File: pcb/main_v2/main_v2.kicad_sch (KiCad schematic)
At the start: 1 part, among them J102 Conn_02x06_Odd_Even

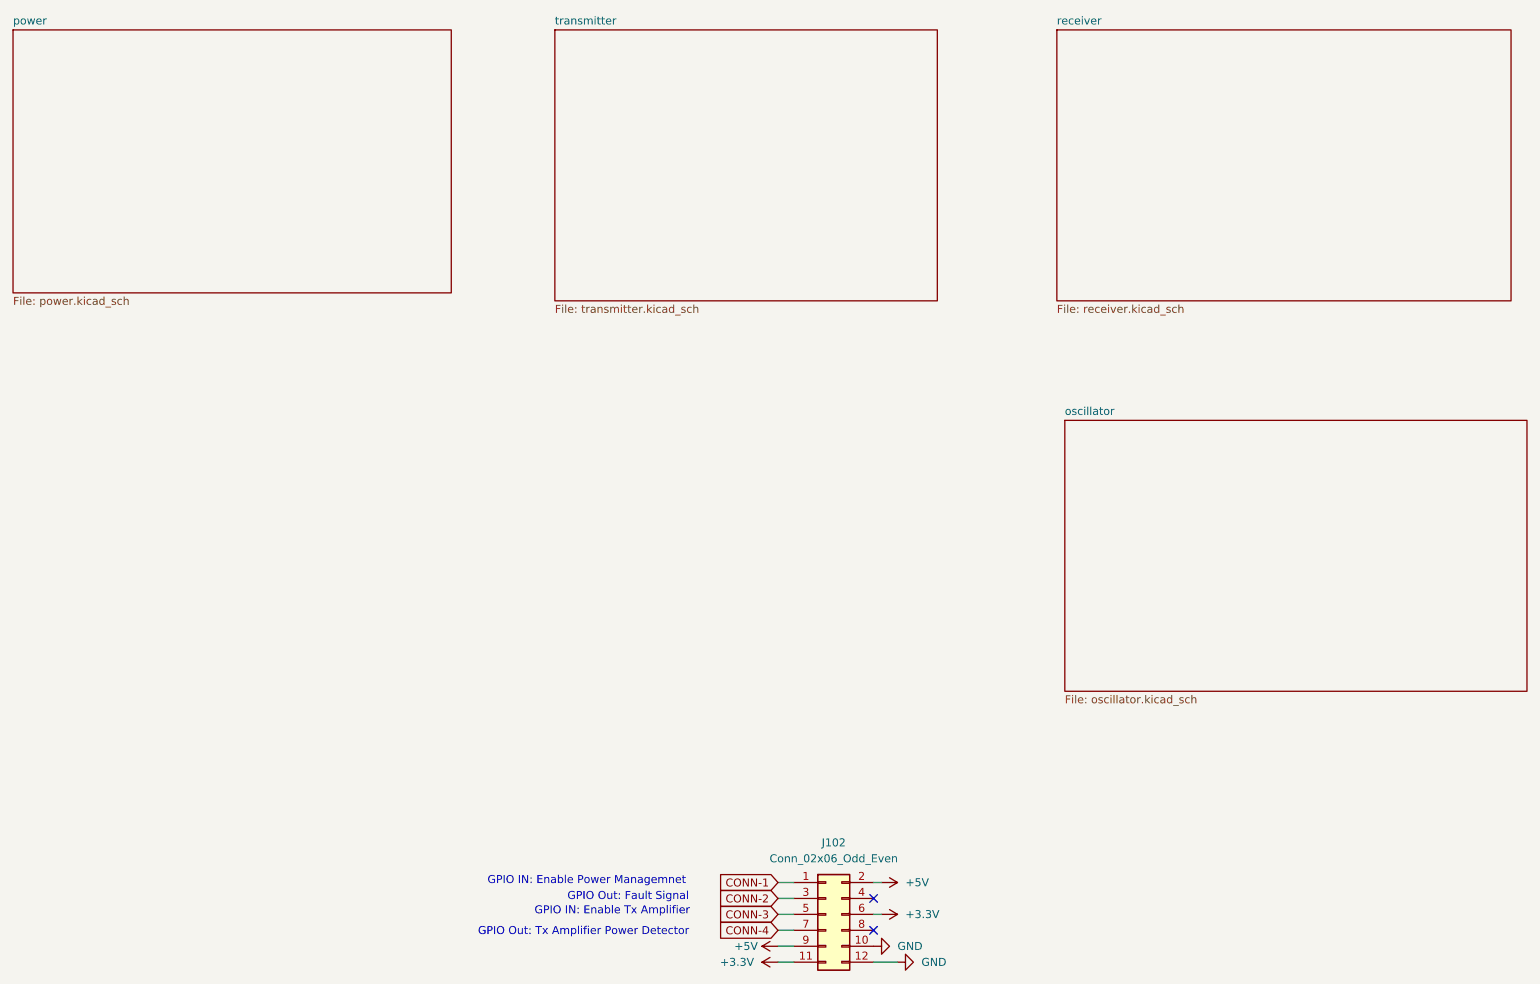
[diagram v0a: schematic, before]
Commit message: updated schematic after review
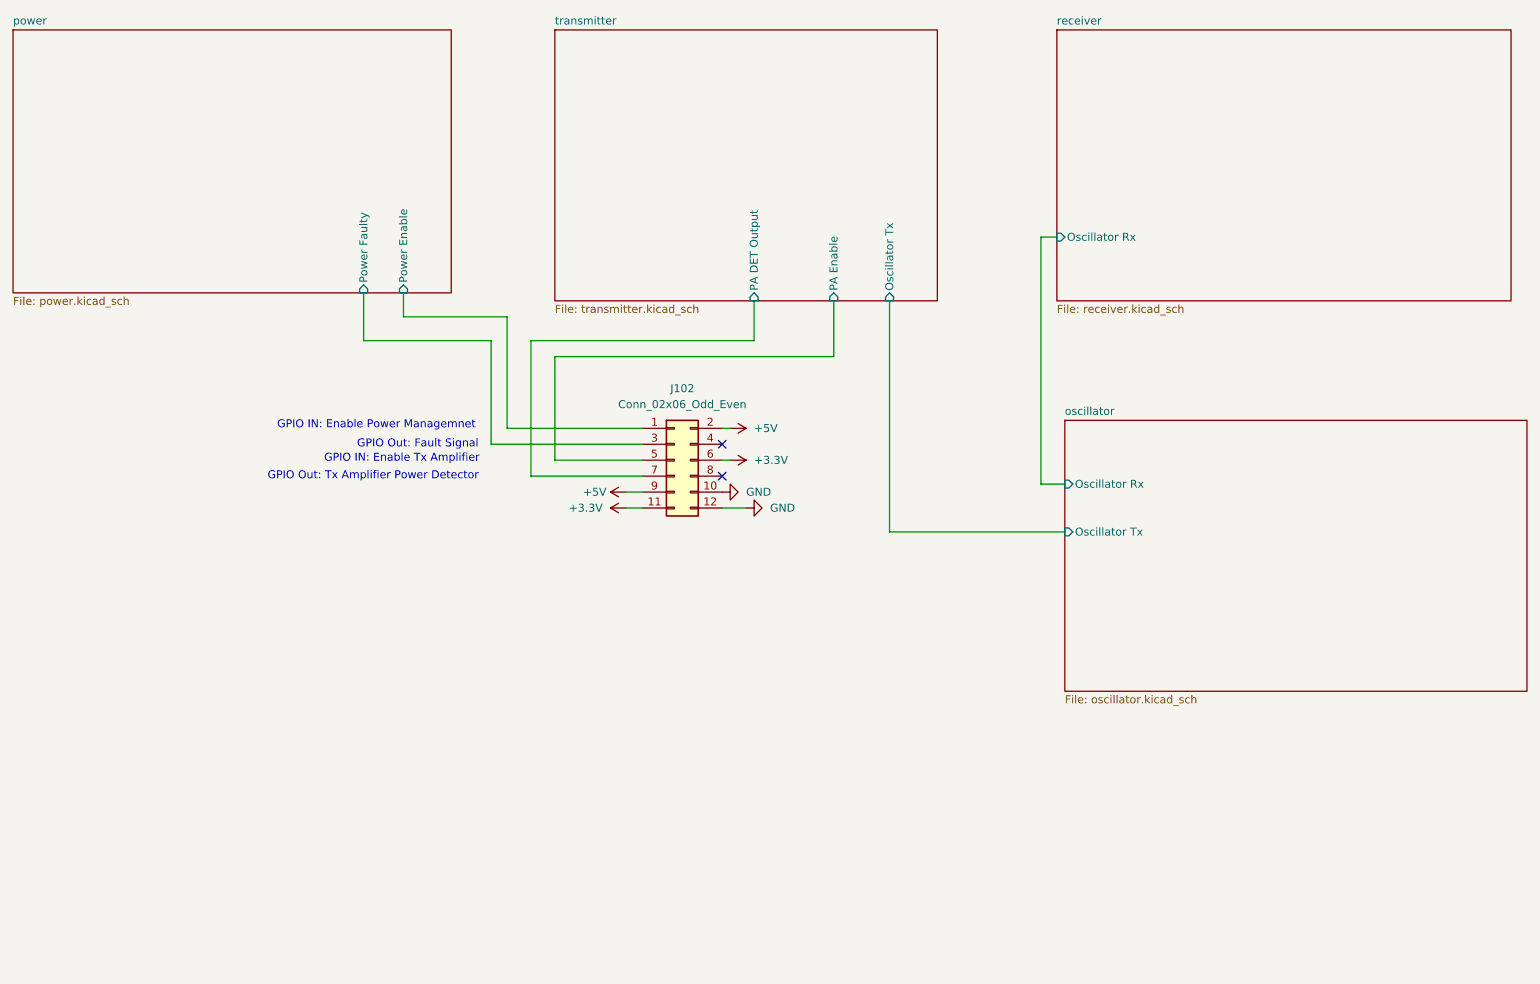
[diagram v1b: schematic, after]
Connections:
- net CONN-1 renamed power/Power Enable
- net CONN-2 renamed power/Power Faulty
- net CONN-3 renamed transmitter/PA Enable
- net CONN-4 renamed transmitter/PA DET Output
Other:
- sheet oscillator ports: added Oscillator Rx, Oscillator Tx; removed none
- sheet power ports: added Power Enable, Power Faulty; removed none
- sheet receiver ports: added Oscillator Rx; removed none
- sheet transmitter ports: added Oscillator Tx, PA DET Output, PA Enable; removed none
- moved on the sheet: J102
